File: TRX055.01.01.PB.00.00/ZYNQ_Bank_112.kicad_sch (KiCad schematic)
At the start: 20 parts, among them J6 Micro_SD_Card, U1 XC7Z015-1CLG485I, U12 USB3320C-EZK-TR, U14 W25Q128JVSIQ

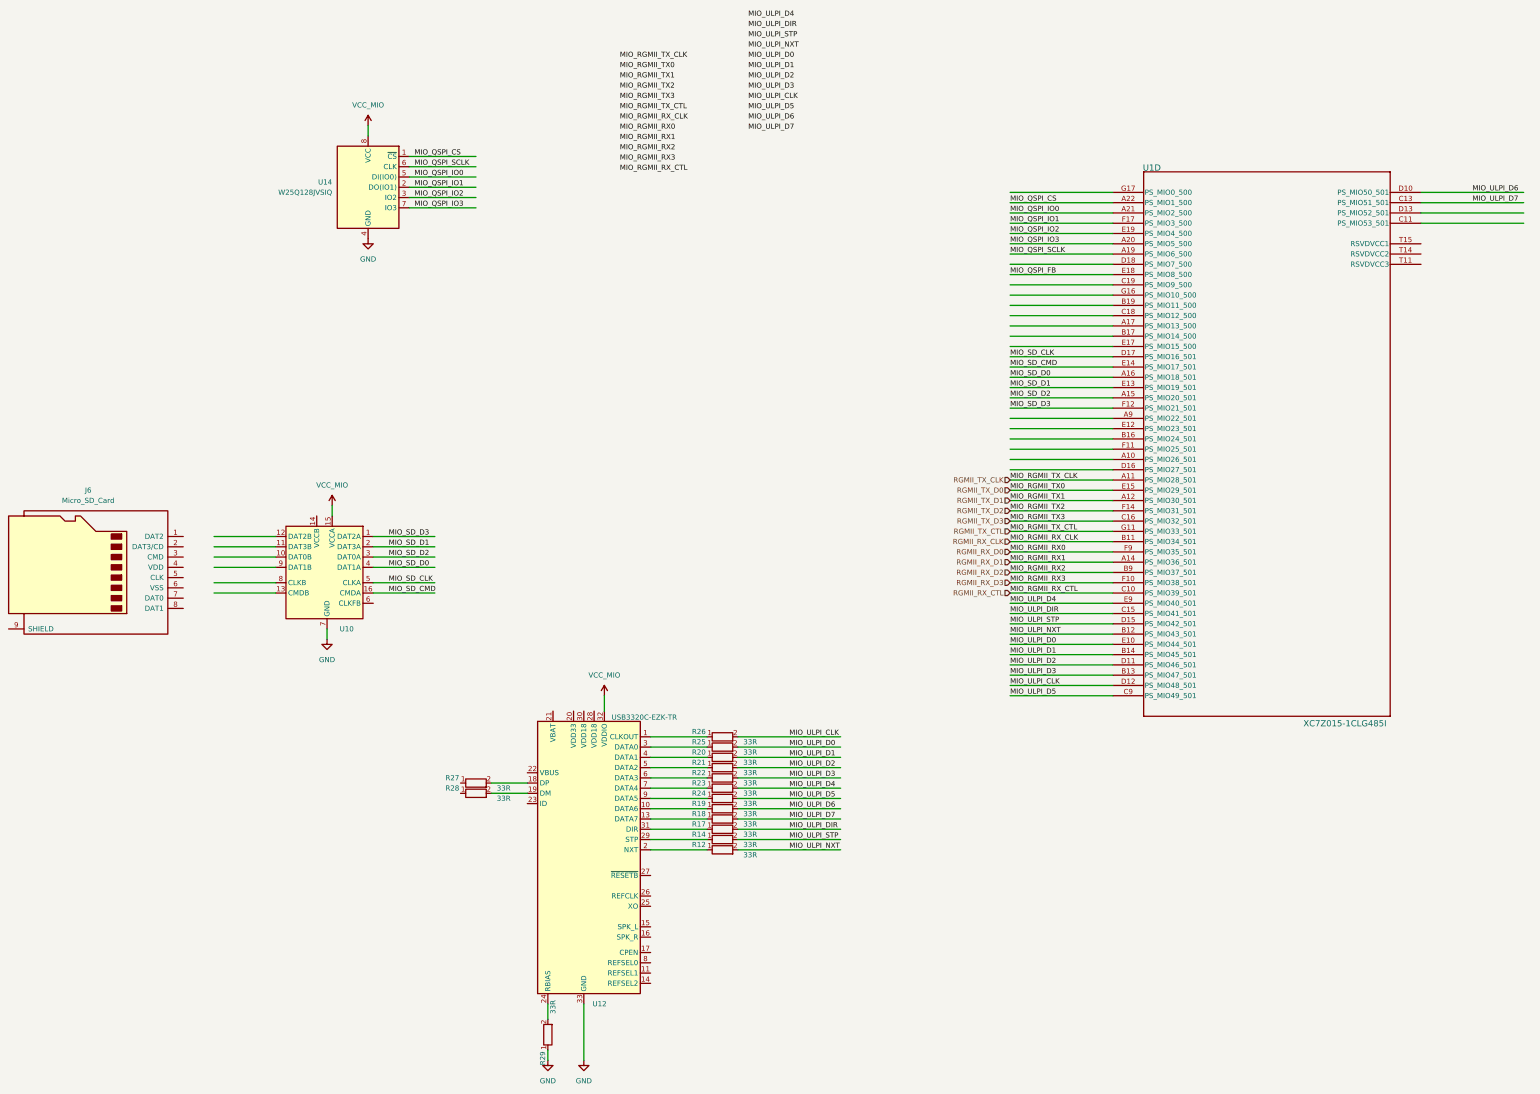
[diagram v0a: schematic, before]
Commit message: Update Layout
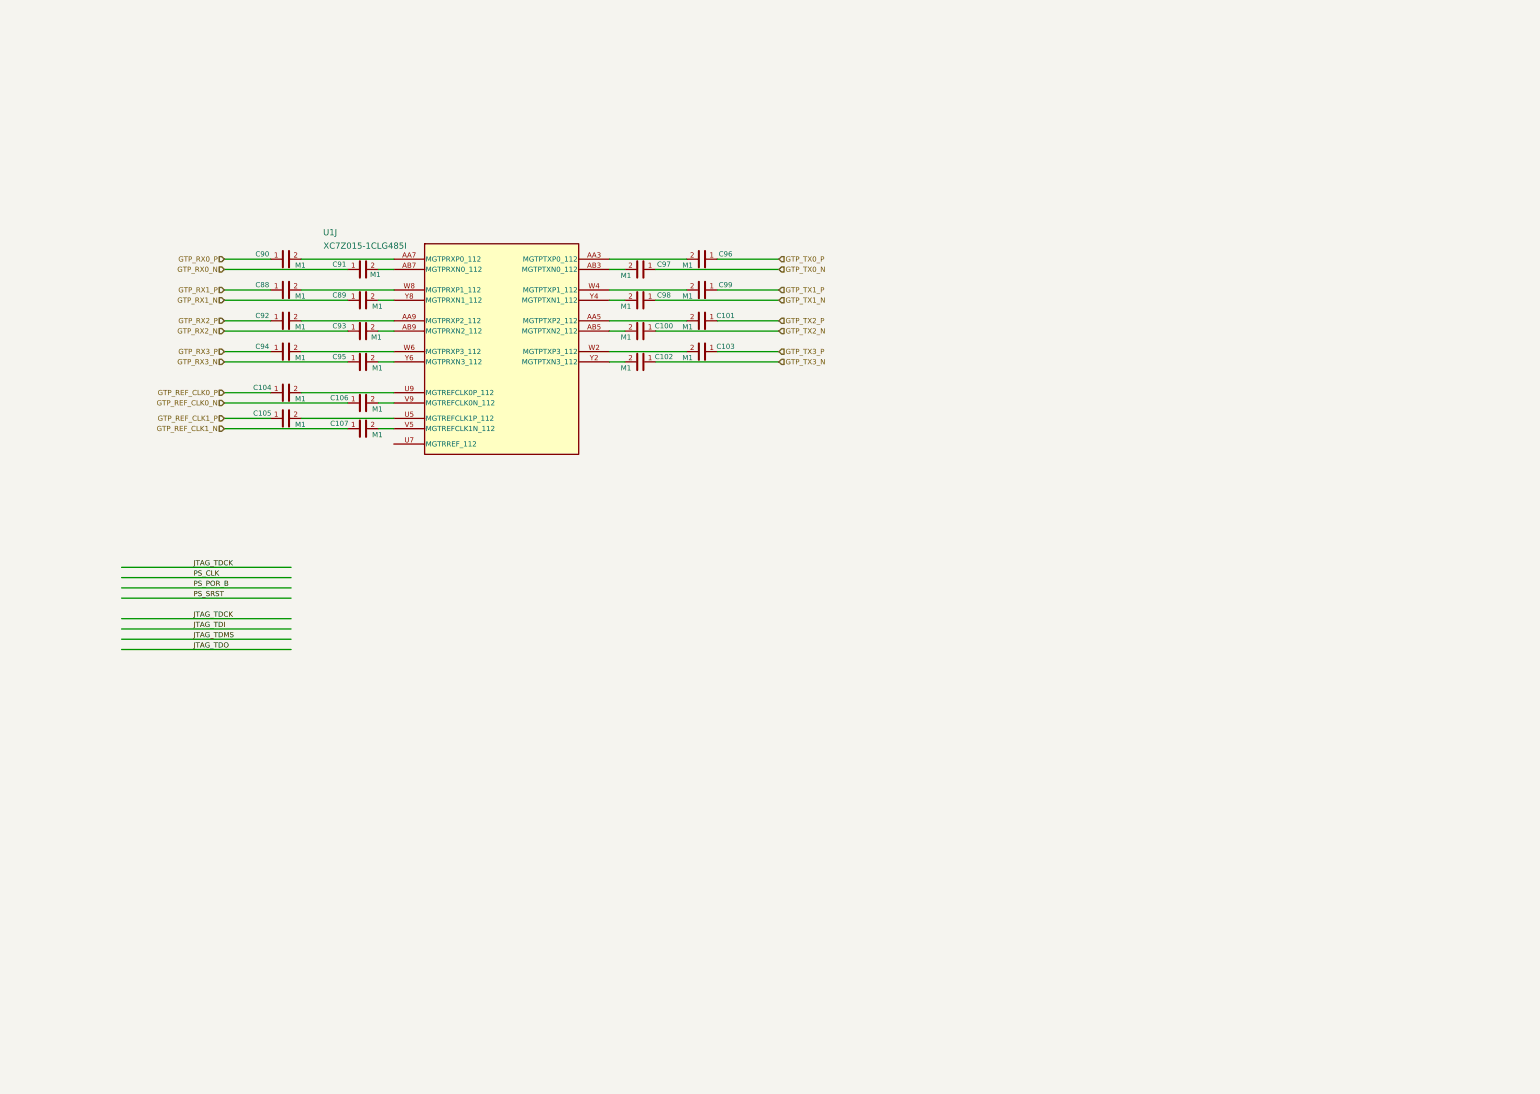
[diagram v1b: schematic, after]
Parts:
- removed J6: Micro_SD_Card, Connector_Card:microSD_HC_Molex_47219-2001, symbol Connector:Micro_SD_Card
- removed R12, R14, R17, R18, R19, R20, R21, R22, R23, R24, R25, R26, R27, R28, R29: 33R, Resistor_SMD:R_0402_1005Metric, symbol PPA-Pasive:Res
- removed U1: XC7Z015-1CLG485I, CLG485XC7Z012S/XC7Z015_AMD, symbol XC7Z015-1CLG485C:XC7Z015-1CLG485I
- removed U10: ~, ppa-active:XQFN16, symbol ppa-ic-com:NVT4858HKZ
- removed U12: USB3320C-EZK-TR, Package_DFN_QFN:QFN-32-1EP_5x5mm_P0.5mm_EP3.3x3.3mm, symbol ppa-ic-com:USB3320C-EZK-TR
- removed U14: W25Q128JVSIQ, Package_SO:SOIC-8_5.23x5.23mm_P1.27mm, symbol Memory_Flash:W25Q128JVS
- added C100, C101, C102, C103, C104, C105, C106, C107, C88, C89, C90, C91, C92, C93, C94, C95, C96, C97, C98, C99: M1, Capacitor_SMD:C_0201_0603Metric, symbol PPA-Pasive:Cap
- added U1: XC7Z015-1CLG485I, CLG485XC7Z012S/XC7Z015_AMD, symbol XC7Z015-1CLG485C:XC7Z015-1CLG485I
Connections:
- new net: C97.2, U1.AB3 (MGTPTXN0_112)
- new net: C101.2, U1.AA5 (MGTPTXP2_112)
- new net: C96.2, U1.AA3 (MGTPTXP0_112)
- new net: C90.2, U1.AA7 (MGTPRXP0_112)
- new net: C92.2, U1.AA9 (MGTPRXP2_112)
- new net: C100.2, U1.AB5 (MGTPTXN2_112)
- new net: C91.2, U1.AB7 (MGTPRXN0_112)
- new net: C93.2, U1.AB9 (MGTPRXN2_112)
- new net: C105.2, U1.U5 (MGTREFCLK1P_112)
- new net: C104.2, U1.U9 (MGTREFCLK0P_112)
- new net: C107.2, U1.V5 (MGTREFCLK1N_112)
- new net: C106.2, U1.V9 (MGTREFCLK0N_112)
- new net: C103.2, U1.W2 (MGTPTXP3_112)
- new net: C99.2, U1.W4 (MGTPTXP1_112)
- new net: C94.2, U1.W6 (MGTPRXP3_112)
- new net: C88.2, U1.W8 (MGTPRXP1_112)
- new net: C102.2, U1.Y2 (MGTPTXN3_112)
- new net: C98.2, U1.Y4 (MGTPTXN1_112)
- new net: C95.2, U1.Y6 (MGTPRXN3_112)
- new net: C89.2, U1.Y8 (MGTPRXN1_112)
- new net GTP_REF_CLK0_N: C106.1
- new net GTP_REF_CLK0_P: C104.1
- new net GTP_REF_CLK1_N: C107.1
- new net GTP_REF_CLK1_P: C105.1
- new net GTP_RX0_N: C91.1
- new net GTP_RX0_P: C90.1
- new net GTP_RX1_N: C89.1
- new net GTP_RX1_P: C88.1
- new net GTP_RX2_N: C93.1
- new net GTP_RX2_P: C92.1
- new net GTP_RX3_N: C95.1
- new net GTP_RX3_P: C94.1
- new net GTP_TX0_N: C97.1
- new net GTP_TX0_P: C96.1
- new net GTP_TX1_N: C98.1
- new net GTP_TX1_P: C99.1
- new net GTP_TX2_N: C100.1
- new net GTP_TX2_P: C101.1
- new net GTP_TX3_N: C102.1
- new net GTP_TX3_P: C103.1
